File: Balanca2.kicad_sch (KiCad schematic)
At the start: 32 parts, among them J1 Conn_01x03_Pin, J2 Conn_01x03_Pin, J3 Conn_01x03_Pin, J4 Conn_01x03_Pin, J5 Conn_01x03_Pin, J6 Conn_01x03, J7 Conn_01x05, Q1 BC547, Q2 BC557, U1 TL082, U2 INA128, U4 LM7805_TO220, U5 LM7905_TO220, U6 CD4066BE, U7 TL082, U8 LM393

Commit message: Atualizacao da versao 3
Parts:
- added C10, C11, C12, C13, C14, C15, C6, C7, C8, C9: 100n, Capacitor_THT:C_Disc_D5.0mm_W2.5mm_P2.50mm, symbol Device:C
- added R5, R6: 10k, Resistor_THT:R_Axial_DIN0207_L6.3mm_D2.5mm_P10.16mm_Horizontal, symbol Device:R
- C2, C3: value C_Polarized -> 1u
- R3: value 22k -> 47k
- RV3: value 50k -> 10K
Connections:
- net +15V: now also C10.1, C12.2, C7.2
- net +5V: now also C14.2, C8.2, R5.2, R6.2
- net -15V: now also C11.1, C13.2, C6.2
- net -5V: now also C15.2, C9.2
- net Controle1: now also R6.1
- net Controle2: now also R5.1
- net GND: now also C10.2, C11.2, C12.1, C13.1, C14.1, C15.1, C6.1, C7.1, C8.1, C9.1
- net at RV3.2, RV3.3: now also U2.8 (Rg); no longer U2.1 (Rg)
- net at RV3.1: now also U2.1 (Rg); no longer U2.8 (Rg)
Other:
- note added: "ALIMENTAÇÃO"
- note added: "ALIMENTAÇÃO CELULA DE CARGA + CONECTORES"
- note added: "AMPLIFICADOR DE GANHO 4,7"
- note added: "AMPLIFICADOR DE INSTRUMENTAÇÃO - GANHO DE 1 A 10000"
- note added: "ZERO CROSSING/CONTROLE DAS CHAVES"
- note removed: "AMPLIFICADOR DE GANHO 2,2"
- note removed: "AMPLIFICADOR DE INSTRUMENTAÇÃO - GANHO DE 163 A 4400"
- note removed: "CONECTORES"
- moved on the sheet: C1, D1, D2, J1, J2, J3, J4, J5, J6, J7, JP5, JP6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

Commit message: Atualizacao de esquematico da placa 3
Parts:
- removed D1, D2: 1N4007, Diode_THT:D_DO-41_SOD81_P10.16mm_Horizontal, symbol Diode:1N4007
- added C16: 33p, Capacitor_THT:C_Disc_D5.0mm_W2.5mm_P2.50mm, symbol Device:C
- added C17: 4,7u, Capacitor_THT:CP_Radial_D5.0mm_P2.50mm, symbol Device:C_Polarized
- added D3, D4: 1N4007, Diode_THT:D_DO-41_SOD81_P10.16mm_Horizontal, symbol Diode:1N4007
- added R10, R11: 100k, Resistor_THT:R_Axial_DIN0207_L6.3mm_D2.5mm_P2.54mm_Vertical, symbol Device:R
- added R12: 10k, Resistor_THT:R_Axial_DIN0207_L6.3mm_D2.5mm_P10.16mm_Horizontal, symbol Device:R
- added R7, R8: 330, Resistor_THT:R_Axial_DIN0207_L6.3mm_D2.5mm_P10.16mm_Horizontal, symbol Device:R
- added R9: 33, Resistor_THT:R_Axial_DIN0207_L6.3mm_D2.5mm_P10.16mm_Horizontal, symbol Device:R
- C1: value 50n -> 470n
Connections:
- net +15V: now also C14.2, U4.1 (VI), U8.8 (V+), D3.1 (K), R11.2, R7.2; no longer J3.1 (Pin_1), J3.2 (Pin_2), J3.3 (Pin_3), Q1.1 (C), RV1.3
- net +5V: no longer C14.2, U8.8 (V+)
- net -15V: now also U5.2 (VI), D4.2 (A), R10.1, R8.1; no longer J2.1 (Pin_1), J2.2 (Pin_2), J2.3 (Pin_3), Q2.1 (C), RV1.1
- net -5V: now also U6.13, U6.5
- net CelulaCargaAlimentacaoV+: now also C16.2, R9.2; no longer Q1.3 (E), Q2.3 (E)
- net GND: now also U1.3 (+), U6.1, U6.2, U6.3, U6.4, C16.1, C17.2; no longer U6.13
- net at C1.1, U7.2 (-): now also R12.2; no longer R1.2, R3.1
- net at U1.1: now also U1.2 (-)
- new net: R10.2, RV1.1
- new net: R11.1, RV1.3
- new net: Q2.1 (C), R8.2
- new net: Q1.3 (E), Q2.3 (E), R9.1
- new net: C17.1, R1.2, R12.1, R3.1
- new net: Q1.1 (C), R7.1
- new net Entrada+15V: D3.2 (A), J3.1 (Pin_1), J3.2 (Pin_2), J3.3 (Pin_3)
- new net Entrada-15V: D4.1 (K), J2.1 (Pin_1), J2.2 (Pin_2), J2.3 (Pin_3)
- no-connect marks 10 -> 2
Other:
- note added: "CAPACITORES E CONEXOES"
- note added: "DEMODULADOR"
- note removed: "CURTOS"
- title: (none) -> Balanca AC
- moved on the sheet: C10, C11, C12, C13, C14, C15, C2, C3, C4, C5, C6, C7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

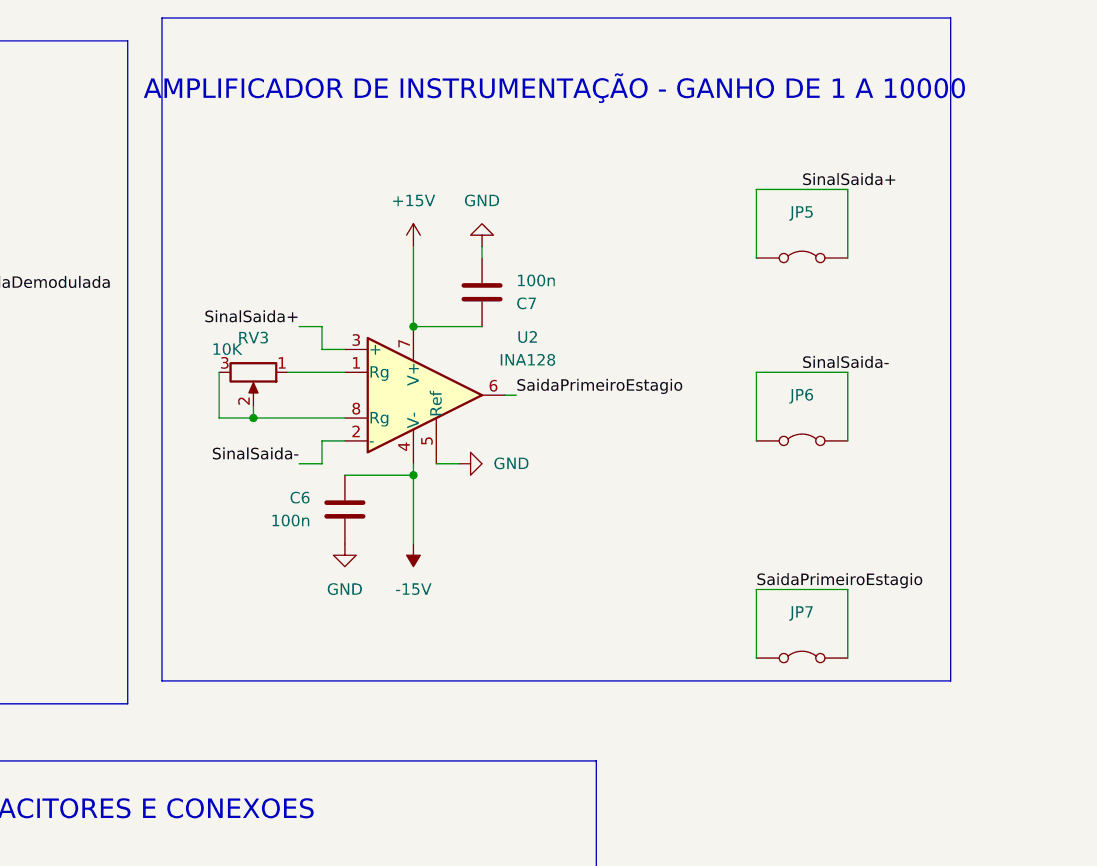
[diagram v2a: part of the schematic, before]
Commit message: Inicio do Roteamento
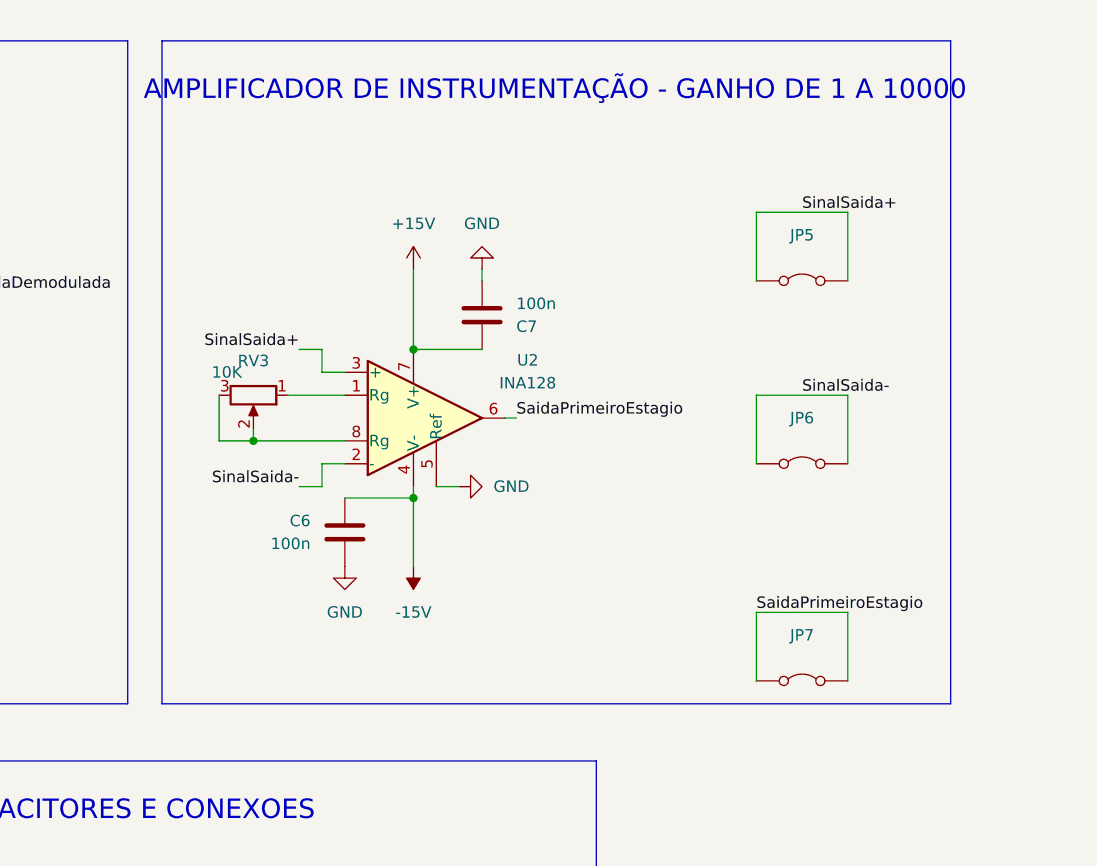
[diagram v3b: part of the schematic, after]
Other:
- moved on the sheet: C6, C7, JP5, JP6, JP7, RV3, U2
